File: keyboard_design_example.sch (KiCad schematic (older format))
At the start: 24 parts, among them SW1 SW_PUSH, U1 ATmega32U4-AU, Y1 16MHz

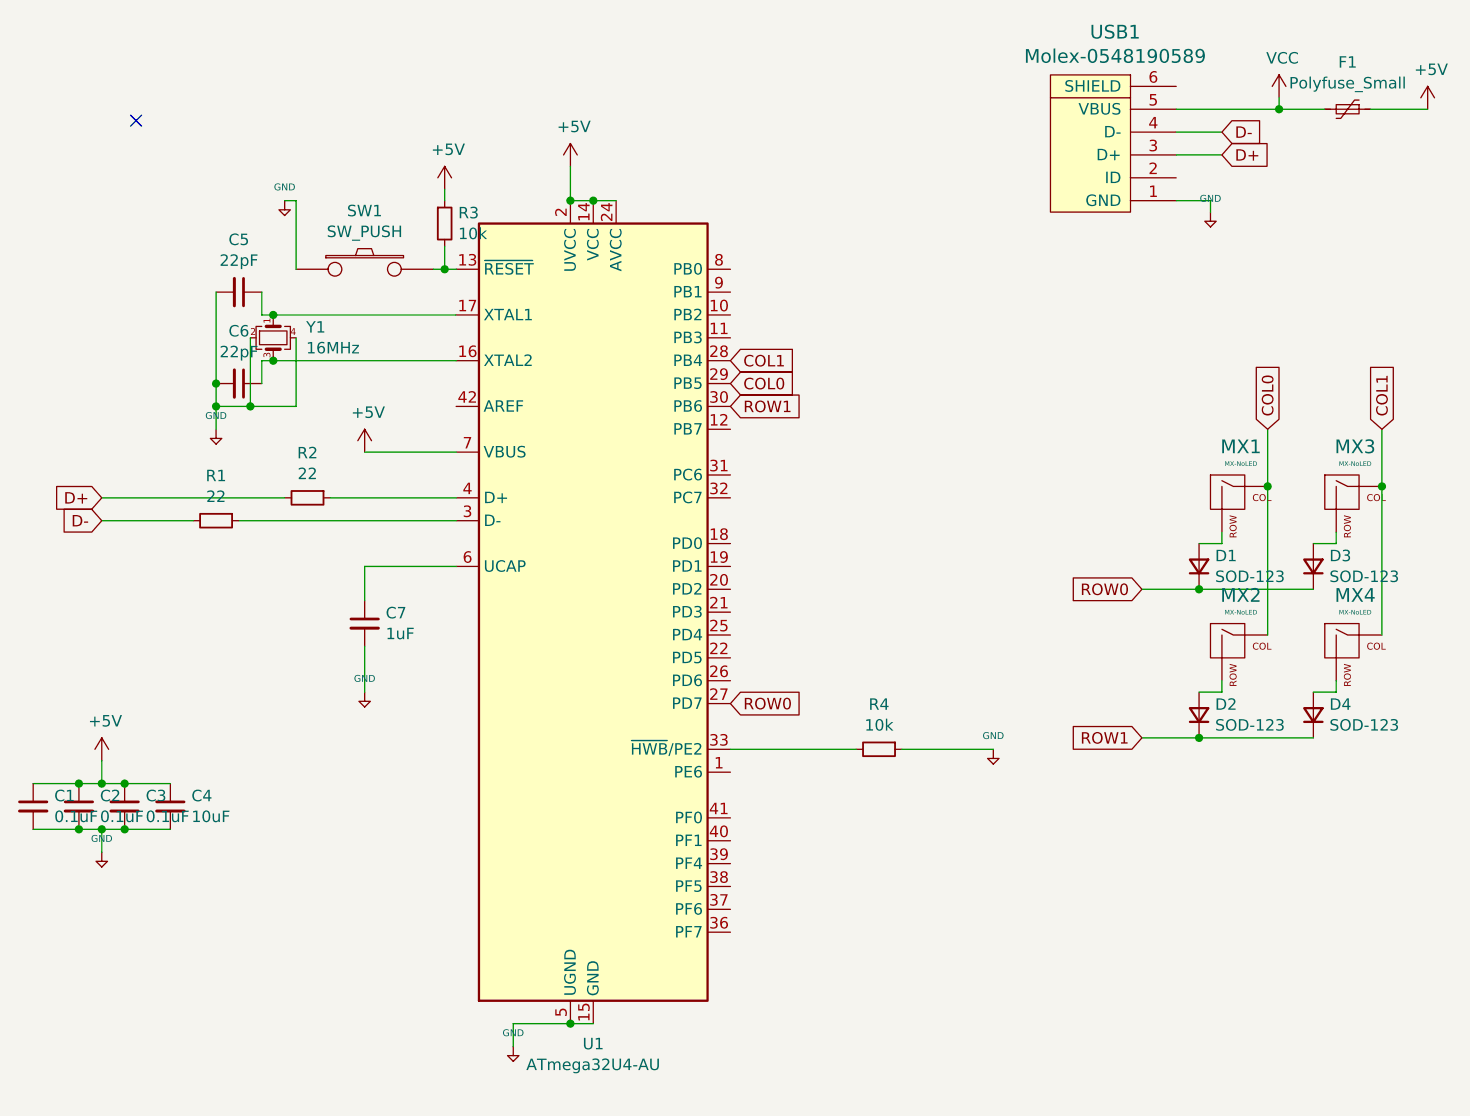
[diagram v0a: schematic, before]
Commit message: Update and work
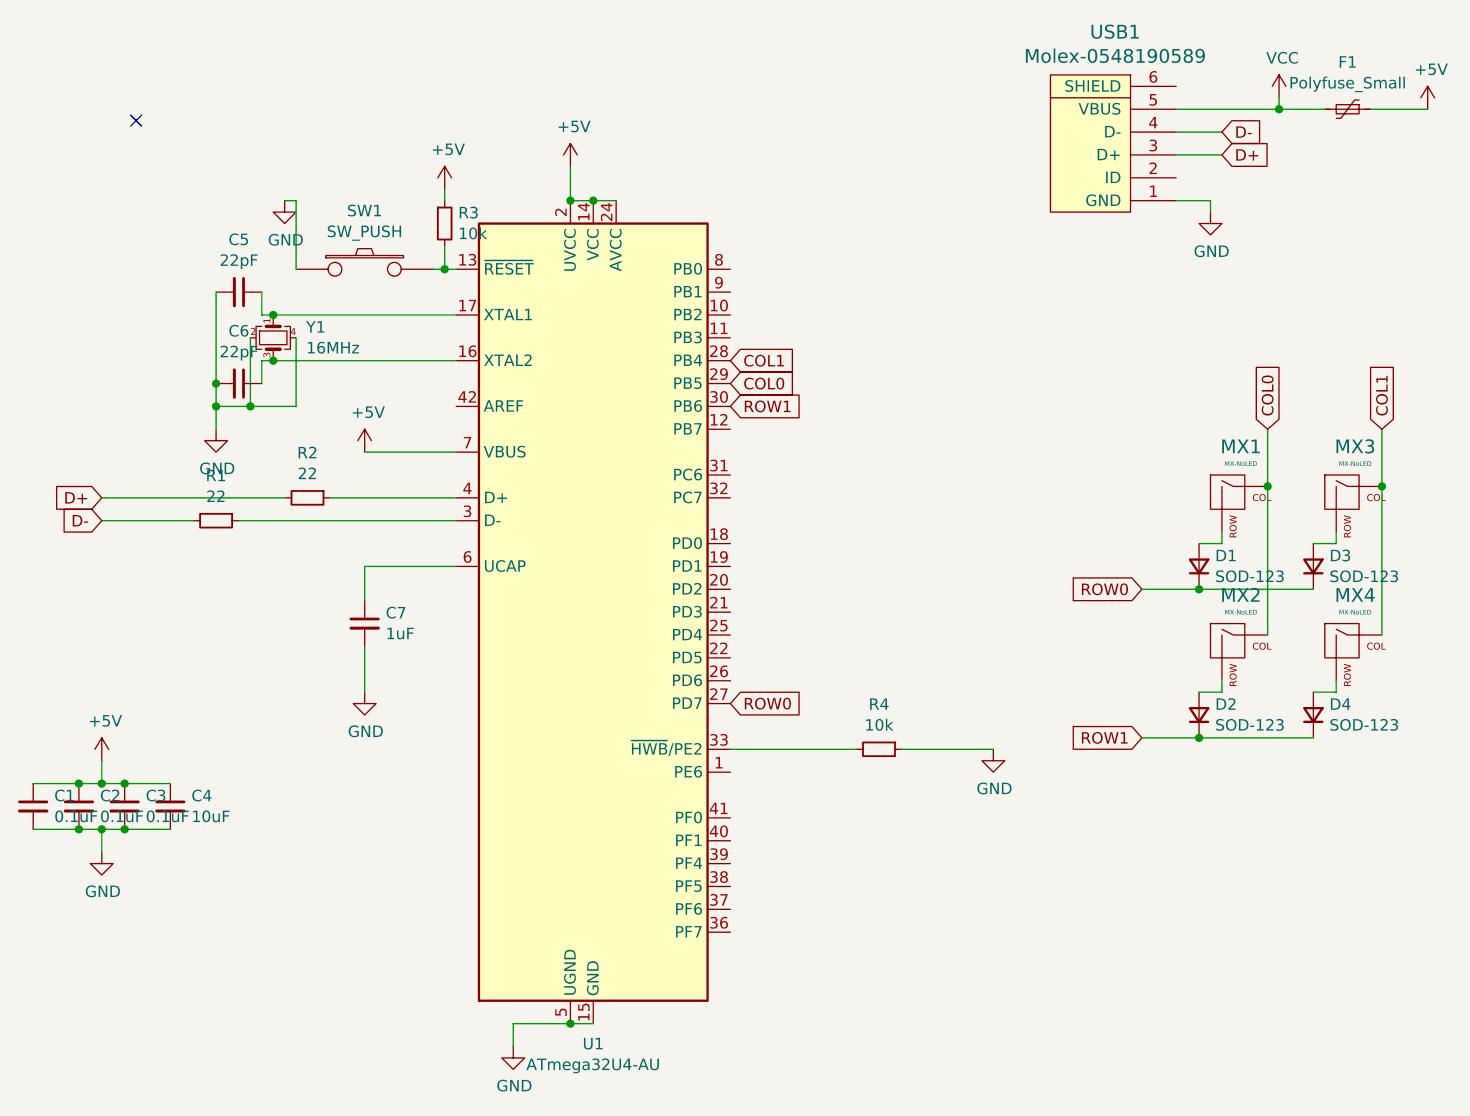
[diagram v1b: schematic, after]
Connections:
- net +5V: no longer C1.2, C2.2, C3.2, C4.2, C5.2, C6.2, C7.2, R4.1, SW1.1, U1.15 (GND), U1.23 (GND), U1.35 (GND), U1.43 (GND), U1.5 (UGND), USB1.1 (GND), Y1.2, Y1.4
- new net GND: C1.2, C2.2, C3.2, C4.2, C5.2, C6.2, C7.2, R4.1, SW1.1, U1.15 (GND), U1.23 (GND), U1.35 (GND), U1.43 (GND), U1.5 (UGND), USB1.1 (GND), Y1.2, Y1.4
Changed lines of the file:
@@
 Wire Wire Line
 	5750 2100 5650 2100
-$Comp
-L keyboard_parts:GND #PWR0102
-U 1 1 60214B8A
-P 5400 5800
-F 0 "#PWR0102" H 5400 5850 20  0001 C CNN
-F 1 "GND" H 5400 5859 30  0000 C CNN
-F 2 "" H 5400 5800 60  0000 C CNN
-F 3 "" H 5400 5800 60  0000 C CNN
-	1    5400 5800
-	1    0    0    -1
-$EndComp
 Wire Wire Line
 	5750 5700 5650 5700
@@
 	0    1    1    0
 $EndComp
-$Comp
-L keyboard_parts:GND #PWR0103
-U 1 1 602192CF
-P 7500 4500
-F 0 "#PWR0103" H 7500 4550 20  0001 C CNN
-F 1 "GND" H 7500 4559 30  0000 C CNN
-F 2 "" H 7500 4500 60  0000 C CNN
-F 3 "" H 7500 4500 60  0000 C CNN
-	1    7500 4500
-	1    0    0    -1
-$EndComp
 Wire Wire Line
 	6350 4500 6900 4500
@@
 Wire Wire Line
 	4750 3700 4750 3850
-$Comp
-L keyboard_parts:GND #PWR0104
-U 1 1 6022339F
-P 4750 4250
-F 0 "#PWR0104" H 4750 4300 20  0001 C CNN
-F 1 "GND" H 4750 4309 30  0000 C CNN
-F 2 "" H 4750 4250 60  0000 C CNN
-F 3 "" H 4750 4250 60  0000 C CNN
-	1    4750 4250
-	1    0    0    -1
-$EndComp
 Wire Wire Line
 	4750 4050 4750 4250
@@
 Wire Wire Line
 	4250 3000 4100 3000
-$Comp
-L keyboard_parts:GND #PWR0106
-U 1 1 60232D3A
-P 4100 3100
-F 0 "#PWR0106" H 4100 3150 20  0001 C CNN
-F 1 "GND" H 4100 3159 30  0000 C CNN
-F 2 "" H 4100 3100 60  0000 C CNN
-F 3 "" H 4100 3100 60  0000 C CNN
-	1    4100 3100
-	1    0    0    -1
-$EndComp
 Wire Wire Line
 	4100 3000 4100 3100
@@
 Wire Wire Line
 	5150 2400 5100 2400
-$Comp
-L keyboard_parts:GND #PWR0107
-U 1 1 6023828E
-P 4400 2100
-F 0 "#PWR0107" H 4400 2150 20  0001 C CNN
-F 1 "GND" H 4400 2159 30  0000 C CNN
-F 2 "" H 4400 2100 60  0000 C CNN
-F 3 "" H 4400 2100 60  0000 C CNN
-	1    4400 2100
-	1    0    0    -1
-$EndComp
 $Comp
 L power:+5V #PWR0108
@@
 F 3 "" H 3600 4550 50  0001 C CNN
 	1    3600 4550
-	1    0    0    -1
-$EndComp
-$Comp
-L keyboard_parts:GND #PWR0110
-U 1 1 60244FF0
-P 3600 4950
-F 0 "#PWR0110" H 3600 5000 20  0001 C CNN
-F 1 "GND" H 3600 5009 30  0000 C CNN
-F 2 "" H 3600 4950 60  0000 C CNN
-F 3 "" H 3600 4950 60  0000 C CNN
-	1    3600 4950
 	1    0    0    -1
 $EndComp
@@
 Wire Wire Line
 	8450 2100 8450 2150
-$Comp
-L keyboard_parts:GND #PWR0113
-U 1 1 602538F7
-P 8450 2150
-F 0 "#PWR0113" H 8450 2200 20  0001 C CNN
-F 1 "GND" H 8450 2209 30  0000 C CNN
-F 2 "" H 8450 2150 60  0000 C CNN
-F 3 "" H 8450 2150 60  0000 C CNN
-	1    8450 2150
-	1    0    0    -1
-$EndComp
 Wire Wire Line
 	8300 1900 8500 1900
@@
 Wire Wire Line
 	4450 2100 4400 2100
+$Comp
+L power:GND #PWR0102
+U 1 1 60242F11
+P 3600 4950
+F 0 "#PWR0102" H 3600 4700 50  0001 C CNN
+F 1 "GND" H 3605 4777 50  0000 C CNN
+F 2 "" H 3600 4950 50  0001 C CNN
+F 3 "" H 3600 4950 50  0001 C CNN
+	1    3600 4950
+	1    0    0    -1
+$EndComp
+$Comp
+L power:GND #PWR0103
+U 1 1 60247D6C
+P 4100 3100
+F 0 "#PWR0103" H 4100 2850 50  0001 C CNN
+F 1 "GND" H 4105 2927 50  0000 C CNN
+F 2 "" H 4100 3100 50  0001 C CNN
+F 3 "" H 4100 3100 50  0001 C CNN
+	1    4100 3100
+	1    0    0    -1
+$EndComp
+$Comp
+L power:GND #PWR0104
+U 1 1 60249D69
+P 4400 2100
+F 0 "#PWR0104" H 4400 1850 50  0001 C CNN
+F 1 "GND" H 4405 1927 50  0000 C CNN
+F 2 "" H 4400 2100 50  0001 C CNN
+F 3 "" H 4400 2100 50  0001 C CNN
+	1    4400 2100
+	1    0    0    -1
+$EndComp
+$Comp
+L power:GND #PWR0106
+U 1 1 6024BCD7
+P 7500 4500
+F 0 "#PWR0106" H 7500 4250 50  0001 C CNN
+F 1 "GND" H 7505 4327 50  0000 C CNN
+F 2 "" H 7500 4500 50  0001 C CNN
+F 3 "" H 7500 4500 50  0001 C CNN
+	1    7500 4500
+	1    0    0    -1
+$EndComp
+$Comp
+L power:GND #PWR0107
+U 1 1 6024DB1C
+P 5400 5800
+F 0 "#PWR0107" H 5400 5550 50  0001 C CNN
+F 1 "GND" H 5405 5627 50  0000 C CNN
+F 2 "" H 5400 5800 50  0001 C CNN
+F 3 "" H 5400 5800 50  0001 C CNN
+	1    5400 5800
+	1    0    0    -1
+$EndComp
+$Comp
+L power:GND #PWR0110
+U 1 1 6024FA6D
+P 4750 4250
+F 0 "#PWR0110" H 4750 4000 50  0001 C CNN
+F 1 "GND" H 4755 4077 50  0000 C CNN
+F 2 "" H 4750 4250 50  0001 C CNN
+F 3 "" H 4750 4250 50  0001 C CNN
+	1    4750 4250
+	1    0    0    -1
+$EndComp
+$Comp
+L power:GND #PWR0113
+U 1 1 60251816
+P 8450 2150
+F 0 "#PWR0113" H 8450 1900 50  0001 C CNN
+F 1 "GND" H 8455 1977 50  0000 C CNN
+F 2 "" H 8450 2150 50  0001 C CNN
+F 3 "" H 8450 2150 50  0001 C CNN
+	1    8450 2150
+	1    0    0    -1
+$EndComp
 $EndSCHEMATC
